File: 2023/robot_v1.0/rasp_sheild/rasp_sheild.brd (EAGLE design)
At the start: 67.3 x 58.1 mm, 14 parts, among them U1 RASPBERRY_PI_4B_4GB

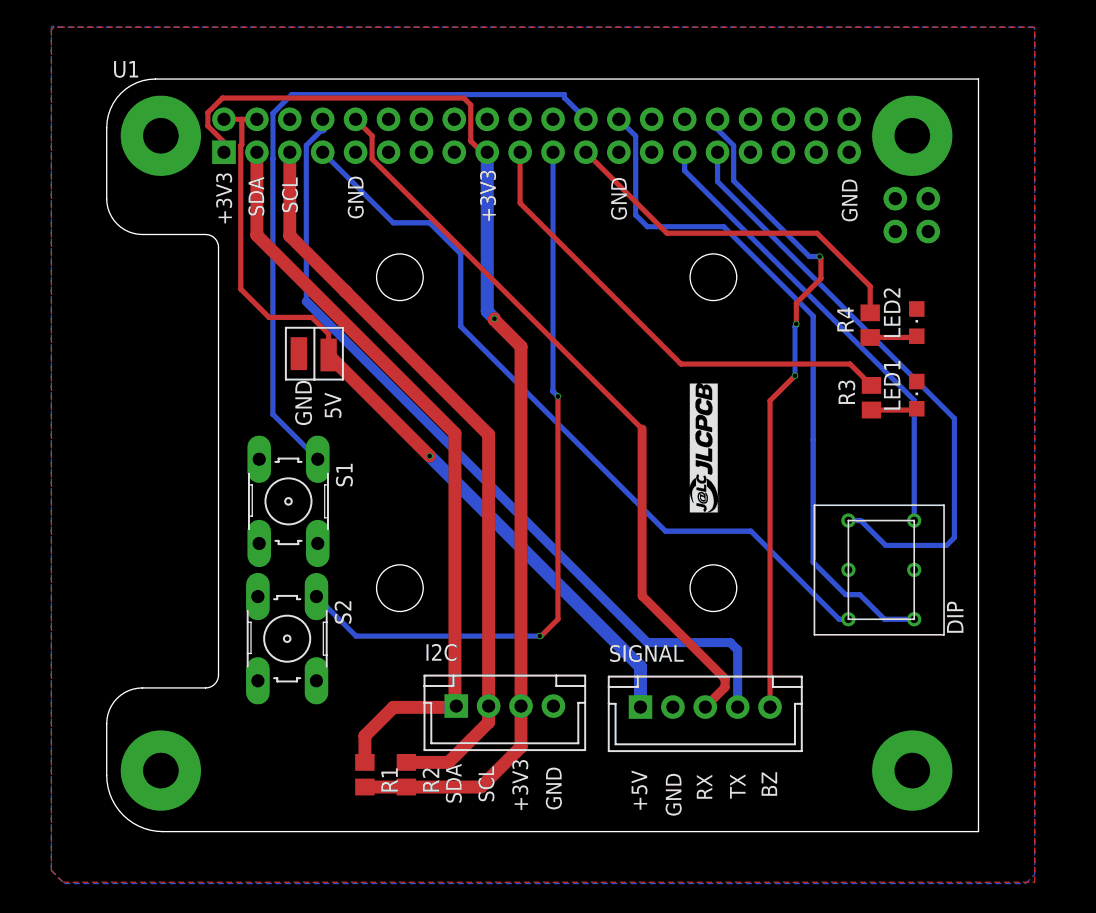
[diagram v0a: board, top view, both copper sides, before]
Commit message: some fix
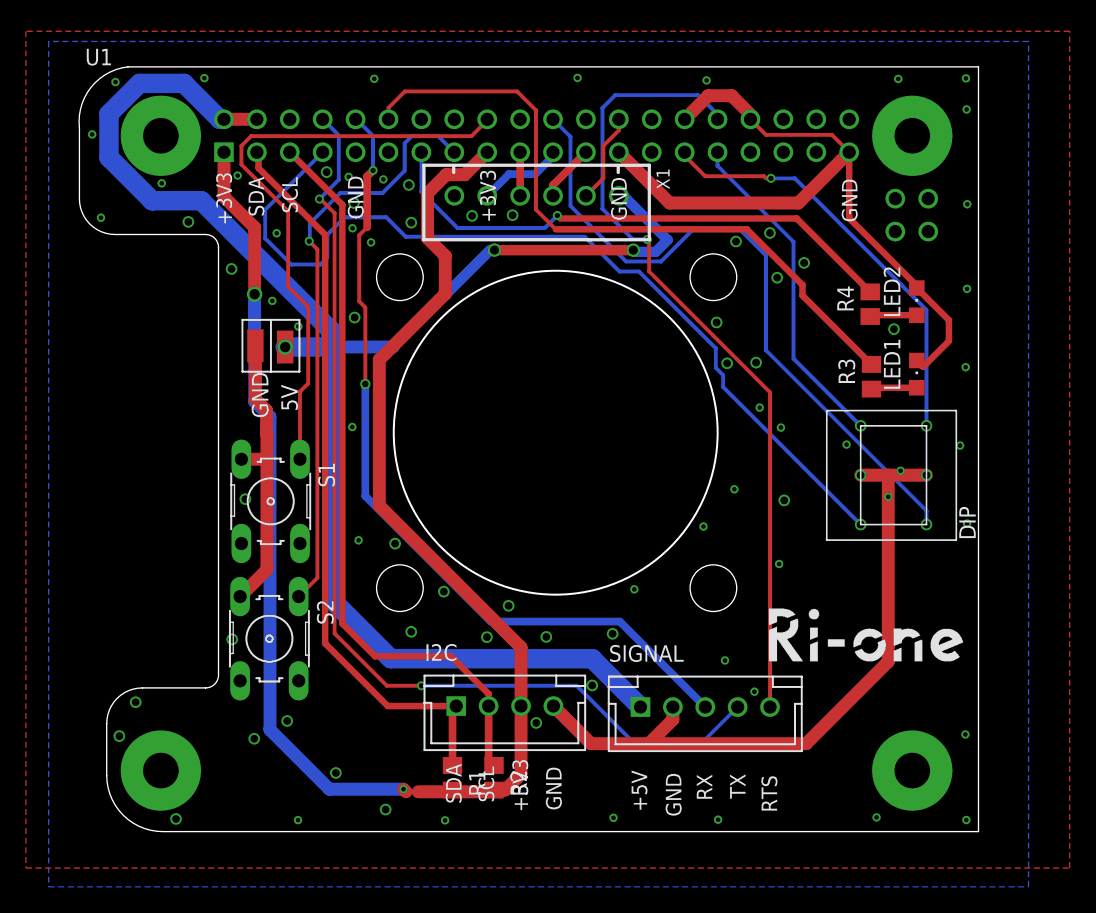
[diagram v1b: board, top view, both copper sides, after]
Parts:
- added X1: JST-XH-06-PIN-ROUND-PAD, JST XH Connectors:JST-XH-06-PACKAGE-ROUND-PAD
- moved DIP 7.37 mm to (63.9, 24.4)
- moved R1 6.77 mm to (27.1, 5.07)
- moved R2 6.77 mm to (30.3, 5.07)
- moved 5V 3.41 mm to (14.1, 38.3)
- moved GND 3.41 mm to (11.8, 38.4)
- moved LED1 1.62 mm to (62.9, 36.2)
- moved R3 1.62 mm to (59.4, 36.0)
- moved R4 1.62 mm to (59.3, 41.6)
- moved LED2 1.62 mm to (62.9, 41.8)
- moved S1 1.37 mm to (13.0, 26.4)
- moved S2 1.37 mm to (12.9, 15.8)
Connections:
- new net CS: U1.26, X1.2
- new net MISO: U1.21, X1.5
- new net MOSI: U1.19, X1.4
- new net SCLK: U1.23, X1.3
- net +5V: now also X1.1
- net GND: now also X1.6
- net LED1: now also U1.12; no longer U1.19
- net LED2: now also U1.13; no longer U1.23
- net R4: now also U1.22; no longer U1.26
- net SW1: now also U1.18; no longer U1.24
- net SW2: now also U1.15; no longer U1.21
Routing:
- net GND: track 0.00 -> 133.4 mm, vias 0 -> 80
- net +5V: track 62.7 -> 125.9 mm, vias 1 -> 3
- net +3V3: track 89.3 -> 128.6 mm, vias 1 -> 2
- net R3: track 46.5 -> 25.7 mm
- net LED1: track 36.9 -> 52.4 mm
- net TX: track 63.4 -> 77.4 mm, vias 0 -> 2
- net LED2: track 28.3 -> 41.7 mm, vias 0 -> 1
- net BZ: track 50.8 -> 62.5 mm, vias 3 -> 1
- net SW2: track 56.7 -> 45.4 mm, vias 2 -> 1
- net R1: track 58.8 -> 69.1 mm
- net SW1: track 53.8 -> 46.5 mm
- net CS: track 0.00 -> 6.95 mm
- net MISO: track 0.00 -> 6.66 mm
- net RX: track 57.8 -> 63.3 mm, vias 0 -> 2
- net SCLK: track 0.00 -> 4.41 mm
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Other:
- board size 67.3 x 58.1 mm -> 69.4 x 59 mm
- board text added: "RTS"
- board text removed: "/Users/mukuyo/Downloads/JLCPCB.BMP.bmp"
- board text removed: "BZ"
